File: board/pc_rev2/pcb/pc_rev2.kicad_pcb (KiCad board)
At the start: 4 copper layers, 200 x 100 mm, 104 parts, among them J1 GND Pins, J2 Conn_01x24, J3 Conn_01x24, J4 Conn_01x05, Q1 SSM3J332R, Q2 BSS138, Q3 BSS138, SW1 SW_Push, SW10 SW_Push, SW11 SW_Push, SW12 SW_Push, SW13 SW_Push, SW14 SW_Push, SW15 SW_Push, SW16 SW_Push, SW17 SW_Push, SW18 SW_Push, SW19 SW_Push, SW2 SW_Push, SW20 SW_Push, SW21 SW_Push, SW22 SW_Push, SW23 SW_Push, SW24 SW_Push, SW25 SW_Push, SW26 SW_Push, SW27 SW_Push, SW28 SW_Push, SW29 SW_Push, SW3 SW_Push, SW30 SW_Push, SW31 SW_Push, SW32 SW_Push, SW33 SW_Push, SW34 SW_Push, SW35 SW_Push, SW36 SW_Push, SW37 SW_Push, SW38 SW_Push, SW39 SW_Push, SW4 SW_Push, SW40 SW_Push, SW41 SW_Push, SW42 SW_Push, SW43 SW_Push, SW44 SW_Push, SW45 SW_Push, SW46 SW_Push, SW47 SW_Push, SW48 SW_Push, SW49 SW_Push, SW5 SW_Push, SW50 SW_Push, SW51 SW_Push, SW52 SW_Push, SW53 SW_Push, SW54 SW_Push, SW55 SW_Push, SW56 SW_Push, SW57 SW_Push, SW58 SW_Push, SW59 SW_Push, SW6 SW_Push, SW60 SW_Push, SW61 SW_Push, SW62 SW_Push, SW63 SW_Push, SW64 SW_Push, SW7 SW_Push, SW8 SW_Push, SW9 SW_Push, U1 AE-FT234X, U2 Tang_nano_9K, U3 SC2004CSWB-XA-LB-G, U4 NJM2742D, U5 4066, U6 TC75S103F, U7 NJU7109, U8 OLED

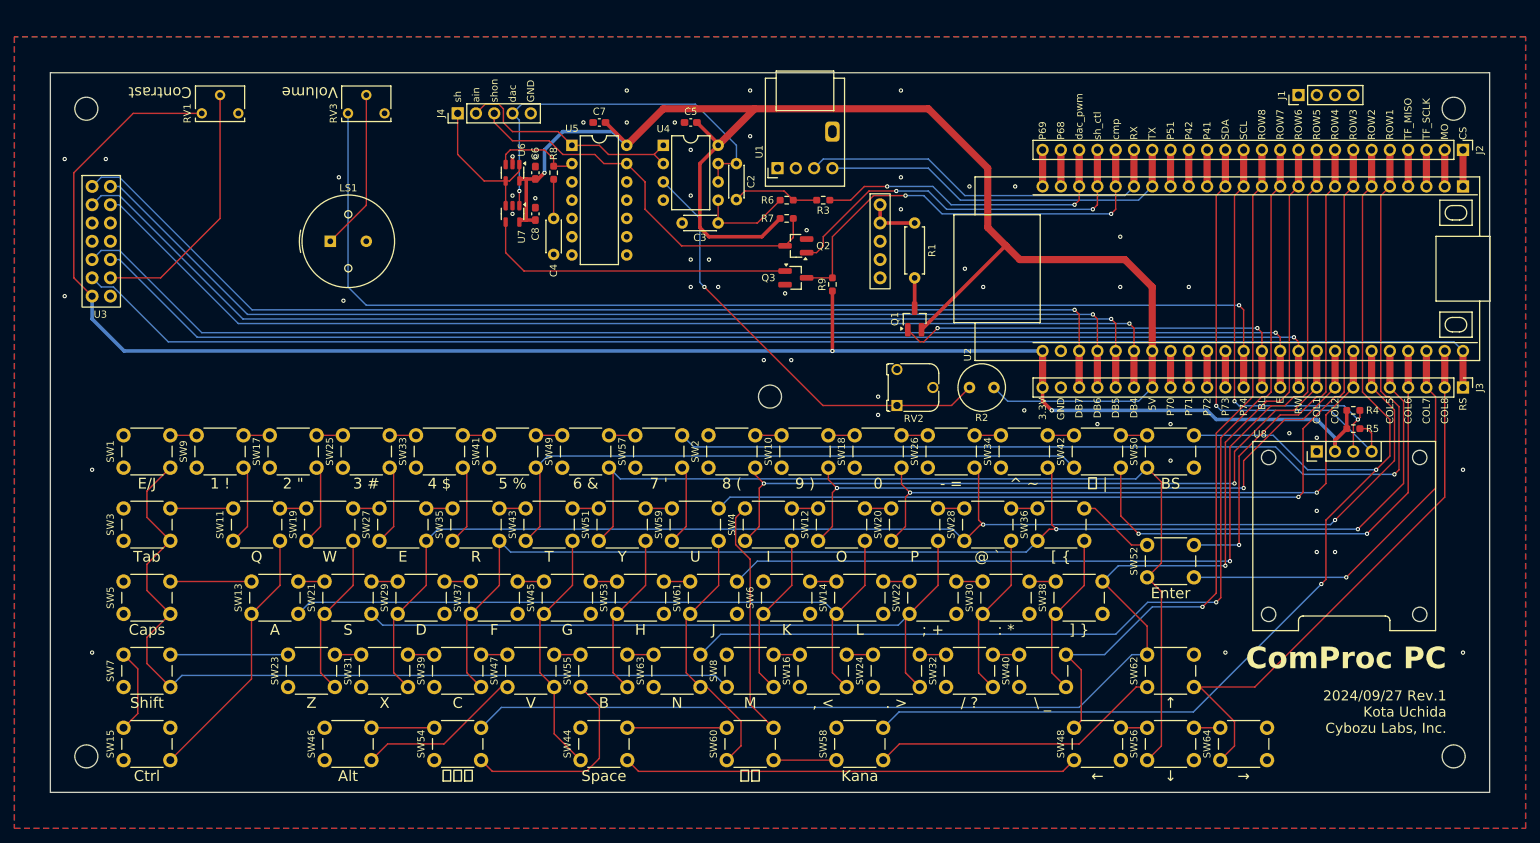
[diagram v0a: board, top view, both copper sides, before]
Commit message: 諸々改良＆基板デザイン（WIP）
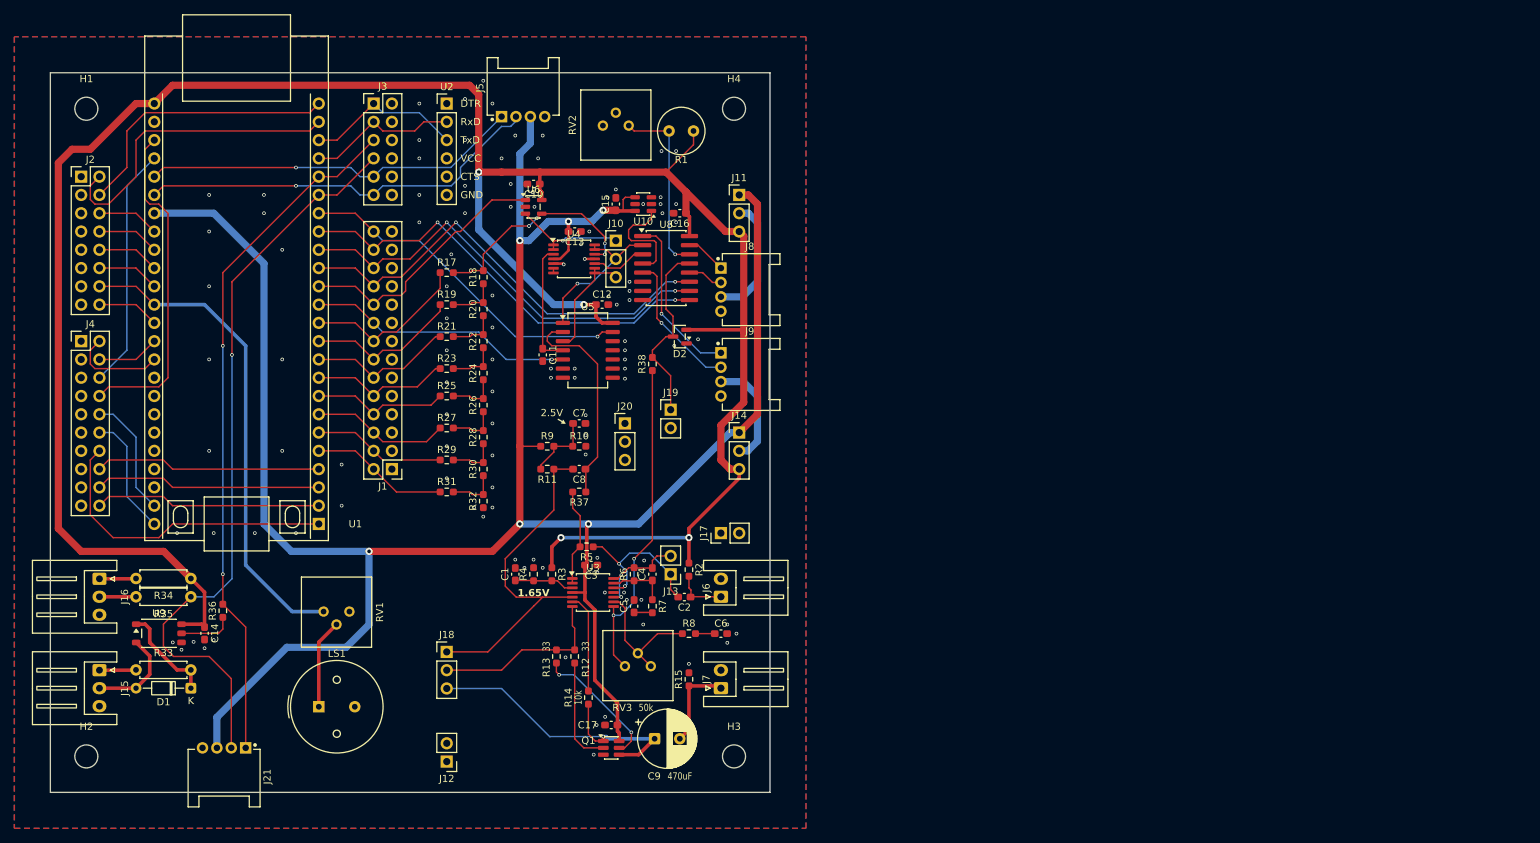
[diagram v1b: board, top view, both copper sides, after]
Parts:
- removed H5: MountingHole, MountingHole:MountingHole_3.2mm_M3
- removed Q2, Q3: BSS138, Package_TO_SOT_SMD:SOT-23_Handsoldering
- removed SW1, SW10, SW11, SW12, SW13, SW14, SW15, SW16, SW17, SW18, SW19, SW2, SW20, SW21, SW22, SW23, SW24, SW25, SW26, SW27, SW28, SW29, SW3, SW30, SW31, SW32, SW33, SW34, SW35, SW36, SW37, SW38, SW39, SW4, SW40, SW41, SW42, SW43, SW44, SW45, SW46, SW47, SW48, SW49, SW5, SW50, SW51, SW52, SW53, SW54, SW55, SW56, SW57, SW58, SW59, SW6, SW60, SW61, SW62, SW63, SW64, SW7, SW8, SW9: SW_Push, Button_Switch_THT:SW_PUSH_6mm_H7.3mm
- removed U7: NJU7109, Package_TO_SOT_SMD:SOT-23-5
- added C1: 100nF, Capacitor_SMD:C_0603_1608Metric_Pad1.08x0.95mm_HandSolder, F.Cu at (109.6, 104.7)
- added C10: 100nF, Capacitor_SMD:C_0603_1608Metric_Pad1.08x0.95mm_HandSolder, F.Cu at (112.1, 50.5)
- added C11: 100pF, Capacitor_SMD:C_0603_1608Metric_Pad1.08x0.95mm_HandSolder, F.Cu at (113.4, 74.2)
- added C12: 100nF, Capacitor_SMD:C_0603_1608Metric_Pad1.08x0.95mm_HandSolder, F.Cu at (121.7, 67.2)
- added C13: 100nF, Capacitor_SMD:C_0603_1608Metric_Pad1.08x0.95mm_HandSolder, F.Cu at (117.9, 57.1)
- added C14: 100n, Capacitor_SMD:C_0603_1608Metric_Pad1.08x0.95mm_HandSolder, F.Cu at (66.4, 112.9)
- added C15: 100nF, Capacitor_SMD:C_0603_1608Metric_Pad1.08x0.95mm_HandSolder, F.Cu at (123.6, 53.2)
- added C16: 100nF, Capacitor_SMD:C_0603_1608Metric_Pad1.08x0.95mm_HandSolder, F.Cu at (132.5, 54.5)
- added C17: 100nF, Capacitor_SMD:C_0603_1608Metric_Pad1.08x0.95mm_HandSolder, F.Cu at (122.9, 125.6)
- added C9: 470uF, Capacitor_THT:CP_Radial_D8.0mm_P3.50mm, F.Cu at (129.0, 127.5)
- added D1: 1N4148, Diode_THT:D_DO-34_SOD68_P7.62mm_Horizontal, F.Cu at (64.5, 120.5)
- added D2: BAT54S, Package_TO_SOT_SMD:SOT-23, F.Cu at (132.5, 71.7)
- added J10: Conn_01x05, Connector_PinHeader_2.54mm:PinHeader_1x03_P2.54mm_Vertical, F.Cu at (123.6, 58.3)
- added J11: Conn_01x03, Connector_PinHeader_2.54mm:PinHeader_1x03_P2.54mm_Vertical, F.Cu at (140.7, 52.0)
- added J12: GND Pins, Connector_PinHeader_2.54mm:PinHeader_1x02_P2.54mm_Vertical, F.Cu at (100.1, 130.7)
- added J13: Conn_01x02, Connector_PinHeader_2.54mm:PinHeader_1x02_P2.54mm_Vertical, F.Cu at (131.2, 104.7)
- added J14: Conn_01x03, Connector_PinHeader_2.54mm:PinHeader_1x03_P2.54mm_Vertical, F.Cu at (140.7, 85.0)
- added J15: INPUT, Connector_JST:JST_XH_S3B-XH-A_1x03_P2.50mm_Horizontal, F.Cu at (51.8, 118.0)
- added J16: OUTPUT, Connector_JST:JST_XH_S3B-XH-A_1x03_P2.50mm_Horizontal, F.Cu at (51.8, 105.3)
- added J17: GND Pins, Connector_PinHeader_2.54mm:PinHeader_1x02_P2.54mm_Vertical, F.Cu at (138.2, 99.0)
- added J18: Conn_01x05, Connector_PinHeader_2.54mm:PinHeader_1x03_P2.54mm_Vertical, F.Cu at (100.1, 115.5)
- added J19: Conn_01x02, Connector_PinHeader_2.54mm:PinHeader_1x02_P2.54mm_Vertical, F.Cu at (131.2, 81.8)
- added J20: Conn_01x03, Connector_PinHeader_2.54mm:PinHeader_1x03_P2.54mm_Vertical, F.Cu at (124.8, 83.7)
- added J21: Conn_Grove_Host, uchan:Grove_1x04_P2mm_THT_Horizontal, F.Cu at (72.1, 128.8)
- added J5: Conn_Grove_Host, uchan:Grove_1x04_P2mm_THT_Horizontal, F.Cu at (107.7, 41.1)
- added J6: Conn_01x03, Connector_JST:JST_XH_S2B-XH-A_1x02_P2.50mm_Horizontal, F.Cu at (138.2, 107.8)
- added J7: Conn_01x03, Connector_JST:JST_XH_S2B-XH-A_1x02_P2.50mm_Horizontal, F.Cu at (138.2, 120.5)
- added J8: Conn_Grove-Analog_Host, uchan:Grove_1x04_P2mm_THT_Horizontal, F.Cu at (138.2, 62.1)
- added J9: Conn_Grove-Analog_Host, uchan:Grove_1x04_P2mm_THT_Horizontal, F.Cu at (138.2, 73.9)
- added R10: 100k, Resistor_SMD:R_0603_1608Metric_Pad0.98x0.95mm_HandSolder, F.Cu at (118.5, 86.9)
- added R11: 100k, Resistor_SMD:R_0603_1608Metric_Pad0.98x0.95mm_HandSolder, F.Cu at (114.0, 90.1)
- added R12: 33, Resistor_SMD:R_0603_1608Metric_Pad0.98x0.95mm_HandSolder, F.Cu at (117.9, 116.1)
- added R13: 33, Resistor_SMD:R_0603_1608Metric_Pad0.98x0.95mm_HandSolder, F.Cu at (115.3, 116.1)
- added R14: 10k, Resistor_SMD:R_0603_1608Metric_Pad0.98x0.95mm_HandSolder, F.Cu at (119.8, 121.8)
- added R15: 10k, Resistor_SMD:R_0603_1608Metric_Pad0.98x0.95mm_HandSolder, F.Cu at (133.7, 119.3)
- added R17: 22k, Resistor_SMD:R_0603_1608Metric_Pad0.98x0.95mm_HandSolder, F.Cu at (100.1, 62.8)
- added R18: 11k, Resistor_SMD:R_0603_1608Metric_Pad0.98x0.95mm_HandSolder, F.Cu at (105.2, 63.4)
- added R19: 22k, Resistor_SMD:R_0603_1608Metric_Pad0.98x0.95mm_HandSolder, F.Cu at (100.1, 67.2)
- added R20: 11k, Resistor_SMD:R_0603_1608Metric_Pad0.98x0.95mm_HandSolder, F.Cu at (105.2, 67.9)
- added R21: 22k, Resistor_SMD:R_0603_1608Metric_Pad0.98x0.95mm_HandSolder, F.Cu at (100.1, 71.7)
- added R22: 11k, Resistor_SMD:R_0603_1608Metric_Pad0.98x0.95mm_HandSolder, F.Cu at (105.2, 72.3)
- added R23: 22k, Resistor_SMD:R_0603_1608Metric_Pad0.98x0.95mm_HandSolder, F.Cu at (100.1, 76.1)
- added R24: 11k, Resistor_SMD:R_0603_1608Metric_Pad0.98x0.95mm_HandSolder, F.Cu at (105.2, 76.7)
- added R25: 22k, Resistor_SMD:R_0603_1608Metric_Pad0.98x0.95mm_HandSolder, F.Cu at (100.1, 79.9)
- added R26: 11k, Resistor_SMD:R_0603_1608Metric_Pad0.98x0.95mm_HandSolder, F.Cu at (105.2, 81.2)
- added R27: 22k, Resistor_SMD:R_0603_1608Metric_Pad0.98x0.95mm_HandSolder, F.Cu at (100.1, 84.4)
- added R28: 11k, Resistor_SMD:R_0603_1608Metric_Pad0.98x0.95mm_HandSolder, F.Cu at (105.2, 85.6)
- added R29: 22k, Resistor_SMD:R_0603_1608Metric_Pad0.98x0.95mm_HandSolder, F.Cu at (100.1, 88.8)
- added R30: 11k, Resistor_SMD:R_0603_1608Metric_Pad0.98x0.95mm_HandSolder, F.Cu at (105.2, 90.1)
- added R31: 22k, Resistor_SMD:R_0603_1608Metric_Pad0.98x0.95mm_HandSolder, F.Cu at (100.1, 93.3)
- added R32: 22k, Resistor_SMD:R_0603_1608Metric_Pad0.98x0.95mm_HandSolder, F.Cu at (105.2, 94.5)
- added R33: 390, uchan:R_Axial_CF25_CFS50_L6.3mm_D2.3mm_P7.62mm_Horizontal, F.Cu at (56.9, 118.0)
- added R34: 33, uchan:R_Axial_CF25_CFS50_L6.3mm_D2.3mm_P7.62mm_Horizontal, F.Cu at (64.5, 105.3)
- added R35: 10, uchan:R_Axial_CF25_CFS50_L6.3mm_D2.3mm_P7.62mm_Horizontal, F.Cu at (64.5, 107.8)
- added R36: 4.7k, Resistor_SMD:R_0603_1608Metric_Pad0.98x0.95mm_HandSolder, F.Cu at (69.0, 109.8)
- added R37: 100k, Resistor_SMD:R_0603_1608Metric_Pad0.98x0.95mm_HandSolder, F.Cu at (118.5, 93.3)
- added R38: 10k, Resistor_SMD:R_0603_1608Metric_Pad0.98x0.95mm_HandSolder, F.Cu at (128.7, 75.5)
- added U10: MCP1501-30xCH, Package_TO_SOT_SMD:SOT-23-6, F.Cu at (127.4, 53.2)
- added U9: TLP2361, Package_SO:SO-5-6_4.55x3.7mm_P1.27mm, F.Cu at (60.1, 112.9)
- C2: value 1.5nF -> 100nF; footprint Capacitor_THT:C_Disc_D4.3mm_W1.9mm_P5.00mm -> Capacitor_SMD:C_0603_1608Metric_Pad1.08x0.95mm_HandSolder
- C3: value 680pF -> 100nF; footprint Capacitor_THT:C_Disc_D4.3mm_W1.9mm_P5.00mm -> Capacitor_SMD:C_0603_1608Metric_Pad1.08x0.95mm_HandSolder
- C4: value 100pF -> 2000pF; footprint Capacitor_THT:C_Disc_D4.3mm_W1.9mm_P5.00mm -> Capacitor_SMD:C_0603_1608Metric_Pad1.08x0.95mm_HandSolder
- C5: value 100nF -> 10uF
- C6: value 100nF -> 1uF
- J1: value GND Pins -> Conn_02x13_Odd_Even; footprint Connector_PinHeader_2.54mm:PinHeader_1x04_P2.54mm_Vertical -> Connector_PinHeader_2.54mm:PinHeader_2x14_P2.54mm_Vertical
- J2: value Conn_01x24 -> Conn_02x08_Row_Letter_Last; footprint Connector_PinHeader_2.54mm:PinHeader_1x24_P2.54mm_Vertical -> Connector_PinHeader_2.54mm:PinHeader_2x08_P2.54mm_Vertical
- J3: value Conn_01x24 -> Conn_02x06_Row_Letter_Last; footprint Connector_PinHeader_2.54mm:PinHeader_1x24_P2.54mm_Vertical -> Connector_PinHeader_2.54mm:PinHeader_2x06_P2.54mm_Vertical
- J4: value Conn_01x05 -> Conn_02x10_Row_Letter_Last; footprint Connector_PinHeader_2.54mm:PinHeader_1x05_P2.54mm_Vertical -> Connector_PinHeader_2.54mm:PinHeader_2x10_P2.54mm_Vertical
- LS1: value PKM13EPYH4000-A0 -> 13mm
- Q1: value SSM3J332R -> BC817BPN; footprint Package_TO_SOT_SMD:SOT-23_Handsoldering -> Package_TO_SOT_SMD:SOT-457T
- R1: value 47 -> 0.5M; footprint Resistor_THT:R_Axial_DIN0207_L6.3mm_D2.5mm_P7.62mm_Horizontal -> OptoDevice:R_LDR_D6.4mm_P3.4mm_Vertical
- R2: value 0.5M -> 2.2k; footprint OptoDevice:R_LDR_D6.4mm_P3.4mm_Vertical -> Resistor_SMD:R_0603_1608Metric_Pad0.98x0.95mm_HandSolder
- R3: value 16k -> 100k
- R4, R5: value 4.7k -> 100k
- R6: value 16k -> 20k
- R7: value 2k -> 200
- R8: value 100 -> 2.2k
- R9: value 2k -> 100k
- RV1: footprint Potentiometer_THT:Potentiometer_Vishay_T73XX_Horizontal -> uchan:Potentiometer_Suntan_TSR-3386K_Vertical
- RV2: footprint uchan:Potentiometer_Suntan_TSR-065_Vertical -> uchan:Potentiometer_Suntan_TSR-3386K_Vertical
- RV3: value 5k -> 50k; footprint Potentiometer_THT:Potentiometer_Vishay_T73XX_Horizontal -> uchan:Potentiometer_Suntan_TSR-3386K_Vertical
- U1: value AE-FT234X -> Tang_nano_9K; footprint uchan:AE-FT234X -> uchan:DIP-48_Tang-Nano-9K
- U2: value Tang_nano_9K -> SKU2782; footprint uchan:DIP-48_Tang-Nano-9K -> uchan:SKU2782
- U3: value SC2004CSWB-XA-LB-G -> LMV324B; footprint uchan:SC2004C_float -> Package_SO:TSSOP-14_4.4x5mm_P0.65mm
- U4: value NJM2742D -> LMV324B; footprint Package_DIP:DIP-8_W7.62mm -> Package_SO:TSSOP-14_4.4x5mm_P0.65mm
- U5: value 4066 -> TC74HC4066AF; footprint Package_DIP:DIP-14_W7.62mm -> Package_SO:SO-14_5.3x10.2mm_P1.27mm
- U6: value TC75S103F -> TPCMP231; footprint Package_TO_SOT_SMD:TSOT-23-5 -> Package_TO_SOT_SMD:SOT-23-5
- U8: value OLED -> 74HC4051; footprint uchan:OLED_Display_I2C -> Package_SO:SOIC-16W_5.3x10.2mm_P1.27mm
- moved H2 210.2 mm to (50.0, 130.0)
- moved J2 192.1 mm to (49.3, 49.4), turned to 0 degrees
- moved J3 156.4 mm to (89.9, 39.3), turned to 0 degrees
- moved U2 141.7 mm to (100.1, 39.3), turned to 0 degrees
- moved J1 136.3 mm to (92.5, 90.1), turned to 180 degrees
- moved H4 134.5 mm to (140.0, 40.0)
- moved R4 116.2 mm to (112.1, 104.7), turned to 90 degrees
- moved R5 107.8 mm to (119.5, 100.9)
- moved U8 93.9 mm to (130.6, 62.1)
- moved H3 90.0 mm to (140.0, 130.0)
- moved RV3 85.2 mm to (126.6, 115.7)
- moved U1 80.7 mm to (82.3, 97.7), turned to 180 degrees
- moved U3 78.7 mm to (120.4, 107.2)
- moved RV1 73.5 mm to (84.8, 111.7), turned to -90 degrees
- moved Q1 73.0 mm to (122.9, 128.8), turned to 0 degrees
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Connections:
- C2 pad 1: Net-(C2-Pad1) -> /audio/mic_in
- C2 pad 2: /ADC/dac_out -> /audio/mic_opin
- C3 pad 2: Net-(U4B-+) -> +5V
- C4 pad 1: Net-(C4-Pad1) -> Net-(U3D--)
- C4 pad 2: GND -> /audio/mic_mid
- C5 pad 1: +5V -> Net-(C5-Pad1)
- C6 pad 1: GND -> Net-(C6-Pad1)
- C6 pad 2: +5V -> GND
- C7 pad 1: +5V -> Net-(C7-Pad1)
- C8 pad 1: +5V -> Net-(C8-Pad1)
- C8 pad 2: GND -> /audio/spk_opin
- J1 pad 2: GND -> /ADC/vref_d0
- J1 pad 4: GND -> /ADC/vref_d1
- J2 pad 1: Net-(J2-Pin_1) -> GND
- J2 pad 10: /ROW6 -> /mcu/gpio4
- J2 pad 11: /ROW7 -> GND
- J2 pad 12: /ROW8 -> /mcu/gpio5
- J2 pad 13: /SCL -> GND
- J2 pad 14: /SDA -> /beep
- J2 pad 15: Net-(J2-Pin_15) -> GND
- J2 pad 16: Net-(J2-Pin_16) -> /mcu/gpio7
- J2 pad 2: Net-(J2-Pin_2) -> /mcu/gpio0
- J2 pad 3: Net-(J2-Pin_3) -> GND
- J2 pad 4: Net-(J2-Pin_4) -> /mcu/gpio1
- J2 pad 5: /ROW1 -> GND
- J2 pad 6: /ROW2 -> /mcu/gpio2
- J2 pad 7: /ROW3 -> GND
- J2 pad 8: /ROW4 -> /mcu/gpio3
- J2 pad 9: /ROW5 -> GND
- J3 pad 1: /RS -> /uart_rx
- J3 pad 10: /RW -> GND
- J3 pad 11: /E -> /sericon_tx
- J3 pad 12: Net-(J3-Pin_12) -> GND
- J3 pad 2: /COL8 -> GND
- J3 pad 3: /COL7 -> /uart_tx
- J3 pad 4: /COL6 -> GND
- J3 pad 5: /COL5 -> /msmp_rx
- J3 pad 6: /COL4 -> GND
- J3 pad 7: /COL3 -> /msmp_tx
- J3 pad 8: /COL2 -> GND
- J3 pad 9: /COL1 -> /sericon_rx
- J4 pad 1: /ADC/sh_buf -> GND
- J4 pad 2: /ADC/ain_buf -> /mcu/dbgio0
- J4 pad 3: /ADC/sh_on_5v -> GND
- J4 pad 4: /ADC/dac_out -> /mcu/dbgio1
- Q1 pad 1: Net-(J3-Pin_12) -> /audio/spk_opout
- Q1 pad 2: +5V -> Net-(Q1A-B1)
- Q1 pad 3: Net-(Q1-D) -> GND
- R1 pad 1: Net-(Q1-D) -> +3.3V
- R1 pad 2: Net-(U3-A) -> /ADC/ain1
- R2 pad 1: +5V -> +3.3V
- R2 pad 2: /ADC/ain -> /audio/mic_in
- R3 pad 1: /adc_dac_pwm -> +3.3V
- R3 pad 2: Net-(C2-Pad1) -> Net-(U3A-+)
- R4 pad 1: /SCL -> Net-(U3A-+)
- R4 pad 2: +3.3V -> GND
- R5 pad 1: /SDA -> /audio/mic_opin
- R5 pad 2: +3.3V -> GNDREF
- R6 pad 1: Net-(C2-Pad1) -> Net-(U3D--)
- R6 pad 2: Net-(U4B-+) -> /audio/mic_mid
- R7 pad 1: +5V -> Net-(U3D--)
- R7 pad 2: /ADC/sh_on_5v -> Net-(C5-Pad1)
- R8 pad 1: Net-(U6-+) -> Net-(U3C--)
- R8 pad 2: Net-(C4-Pad1) -> Net-(C6-Pad1)
- R9 pad 1: +3.3V -> +5V
- R9 pad 2: /adc_cmp -> Net-(C7-Pad1)
- RV1 pad 1: +3.3V -> /beep
- RV1 pad 2: Net-(U3-VO) -> Net-(LS1-Pad1)
- RV2 pad 1: /ADC/ain -> /ADC/ain1
- RV3 pad 1: Net-(J3-Pin_13) -> Net-(U3C--)
- RV3 pad 2: Net-(LS1-Pad1) -> Net-(U3C--)
- RV3 pad 3: GND -> Net-(R38-Pad1)
- U1 pad 1: unconnected-(U1-5V-Pad1) -> /mcu/tf_cs
- U1 pad 2: GND -> /mcu/tf_mosi
- U1 pad 3: /RX -> /mcu/tf_sclk
- U1 pad 4: /TX -> /mcu/tf_miso
- U1 pad 5: unconnected-(U1-CB0-Pad5) -> /ADC/vref_d0
- U2 pad 1: Net-(J2-Pin_1) -> unconnected-(U2-DTR-Pad1)
- U2 pad 2: Net-(J2-Pin_2) -> /uart_tx
- U2 pad 3: Net-(J2-Pin_3) -> /uart_rx
- U2 pad 4: Net-(J2-Pin_4) -> unconnected-(U2-VCC-Pad4)
- U2 pad 5: /ROW1 -> unconnected-(U2-CTS-Pad5)
- U2 pad 6: /ROW2 -> GND
- U3 pad 1: GND -> GNDREF
- U3 pad 10: unconnected-(U3-DB3-Pad10) -> /audio/mic_mid
- U3 pad 11: /DB4 -> GND
- U3 pad 12: /DB5 -> /audio/mic_opin
- U3 pad 13: /DB6 -> Net-(U3D--)
- U3 pad 14: /DB7 -> /audio/mic_mid
- U3 pad 2: +3.3V -> GNDREF
- U3 pad 3: Net-(U3-VO) -> Net-(U3A-+)
- U3 pad 4: /RS -> +5V
- U3 pad 5: /RW -> /audio/spk_opin
- U3 pad 6: /E -> Net-(U3B--)
- U3 pad 7: unconnected-(U3-DB0-Pad7) -> /audio/spk_mid
- U3 pad 8: unconnected-(U3-DB1-Pad8) -> Net-(R38-Pad1)
- U3 pad 9: unconnected-(U3-DB2-Pad9) -> Net-(U3C--)
- U4 pad 1: /ADC/ain_buf -> /ADC/sh_buf
- U4 pad 2: /ADC/ain_buf -> /ADC/sh_buf
- U4 pad 3: /ADC/ain -> Net-(U4A-+)
- U4 pad 4: GND -> +5V
- U4 pad 5: Net-(U4B-+) -> GND
- U4 pad 6: /ADC/dac_out -> Net-(U4B--)
- U4 pad 7: /ADC/dac_out -> Net-(U4B--)
- U4 pad 8: +5V -> /ADC/ain_buf
- U5 pad 1: /ADC/ain_buf -> /ADC/dac_out
- U5 pad 10: unconnected-(U5-Pad10) -> GND
- U5 pad 11: unconnected-(U5-Pad11) -> GND
- U5 pad 13: /ADC/sh_on_5v -> /audio/spk_on
- U5 pad 14: +5V -> +3.3V
- U5 pad 2: Net-(U6-+) -> Net-(C8-Pad1)
- U5 pad 3: unconnected-(U5-Pad3) -> /ADC/ain_buf
- U5 pad 4: unconnected-(U5-Pad4) -> Net-(U4A-+)
- U5 pad 5: GND -> /ADC/sh_on
- U5 pad 8: unconnected-(U5-Pad8) -> GND
- U5 pad 9: unconnected-(U5-Pad9) -> GND
- U6 pad 1: /ADC/sh_buf -> /ADC/cmp
- U6 pad 3: Net-(U6-+) -> /ADC/sh_buf
- U6 pad 4: /ADC/sh_buf -> /ADC/dac_raw
- U6 pad 5: +5V -> +3.3V
- U8 pad 1: GND -> /ADC/ain4
- U8 pad 2: +3.3V -> /ADC/dac_out
- U8 pad 3: /SCL -> Net-(U4C-+)
- U8 pad 4: /SDA -> Net-(U10-OUT)
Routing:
- net /COL6: track 330.2 -> 0.00 mm, vias 2 -> 0
- net /COL1: track 294.0 -> 0.00 mm, vias 2 -> 0
- net /COL7: track 293.3 -> 0.00 mm, vias 1 -> 0
- net /COL2: track 293.2 -> 0.00 mm, vias 2 -> 0
- net /COL3: track 275.4 -> 0.00 mm, vias 2 -> 0
- net /COL4: track 274.7 -> 0.00 mm, vias 2 -> 0
- net /COL5: track 267.7 -> 0.00 mm, vias 2 -> 0
- net /ROW6: track 266.0 -> 0.00 mm, vias 1 -> 0
- net /ROW7: track 240.1 -> 0.00 mm, vias 1 -> 0
- net /ROW2: track 236.8 -> 0.00 mm, vias 2 -> 0
- net /COL8: track 229.6 -> 0.00 mm
- net /ROW1: track 226.0 -> 0.00 mm, vias 1 -> 0
- net /ROW5: track 218.9 -> 0.00 mm, vias 1 -> 0
- net /ROW3: track 215.7 -> 0.00 mm, vias 1 -> 0
- net /RS: track 199.8 -> 0.00 mm
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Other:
- board size 200 x 100 mm -> 100 x 100 mm
- copper layers 4 -> 2
- board text added: "1.65V"
- board text added: "10k"
- board text added: "2.5V"
- board text added: "33"
- board text added: "470uF"
- board text added: "50k"
- board text removed: ", <"
- board text removed: "- ="
- board text removed: ". >"
- board text removed: "/ ?"
- board text removed: "0"
- board text removed: "1 !"
- board text removed: "2 {dblquote}"
- board text removed: "2024/09/27 Rev.1 Kota Uchida Cybozu Labs, Inc."
- board text removed: "3 #"
- board text removed: "3.3V"
- board text removed: "4 $"
- board text removed: "5 %"
- board text removed: "5V"
- board text removed: "6 &"
- board text removed: "7 '"
- board text removed: "8 ("
- board text removed: "9 )"
- board text removed: ": *"
- board text removed: "; +"
- board text removed: "@ `"
- board text removed: "A"
- board text removed: "Alt"
- board text removed: "B"
- board text removed: "BL"
- board text removed: "BS"
- board text removed: "C"
- board text removed: "COL1"
- board text removed: "COL2"
- board text removed: "COL5"
- board text removed: "COL6"
- board text removed: "COL7"
- board text removed: "COL8"
- board text removed: "CS"
- board text removed: "Caps"
- board text removed: "ComProc PC"
- board text removed: "Contrast"
- board text removed: "Ctrl"
- board text removed: "D"
- board text removed: "DB4"
- board text removed: "DB5"
- board text removed: "DB6"
- board text removed: "DB7"
- board text removed: "E"
- board text removed: "E/J"
- board text removed: "Enter"
- board text removed: "F"
- board text removed: "G"
- board text removed: "GND"
- board text removed: "H"
- board text removed: "I"
- board text removed: "J"
- board text removed: "JLCJLCJLCJLC"
- board text removed: "K"
- board text removed: "Kana"
- board text removed: "L"
- board text removed: "M"
- board text removed: "MO"
- board text removed: "N"
- board text removed: "O"
- board text removed: "P"
- board text removed: "P41"
- board text removed: "P42"
- board text removed: "P51"
- board text removed: "P68"
- board text removed: "P69"
- board text removed: "P70"
- board text removed: "P71"
- board text removed: "P72"
- board text removed: "P73"
- board text removed: "P74"
- board text removed: "Q"
- board text removed: "R"
- board text removed: "ROW1"
- board text removed: "ROW2"
- board text removed: "ROW3"
- board text removed: "ROW4"
- board text removed: "ROW5"
- board text removed: "ROW6"
- board text removed: "ROW7"
- board text removed: "ROW8"
- board text removed: "RS"
- board text removed: "RW"
- board text removed: "RX"
- board text removed: "S"
- board text removed: "SCL"
- board text removed: "SDA"
- board text removed: "Shift"
- board text removed: "Space"
- board text removed: "T"
- board text removed: "TF_MISO"
- board text removed: "TF_SCLK"
- board text removed: "TX"
- board text removed: "Tab"
- board text removed: "U"
- board text removed: "V"
- board text removed: "Volume"
- board text removed: "W"
- board text removed: "X"
- board text removed: "Y"
- board text removed: "Z"
- board text removed: "[ {"
- board text removed: "\ _"
- board text removed: "] }"
- board text removed: "^ ~"
- board text removed: "ain"
- board text removed: "cmp"
- board text removed: "dac"
- board text removed: "dac_pwm"
- board text removed: "sh"
- board text removed: "sh_ctl"
- board text removed: "shon"
- board text removed: "←"
- board text removed: "↑"
- board text removed: "→"
- board text removed: "↓"
- board text removed: "変換"
- board text removed: "無変換"
- board text removed: "￥ |"
